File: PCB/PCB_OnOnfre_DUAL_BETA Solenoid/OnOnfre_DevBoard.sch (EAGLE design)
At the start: 31 parts, among them J1 9PIN 2.54MM, J3Y S8050, J7 8p, K1 G5Q-1-DC12, K2 G5Q-1-DC12, U2 esp12

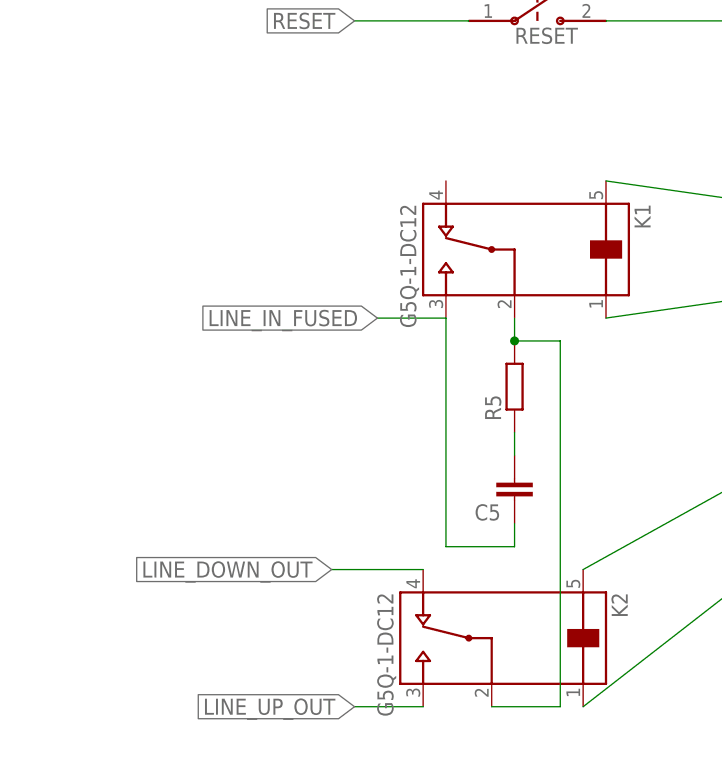
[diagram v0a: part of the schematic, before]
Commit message: estores
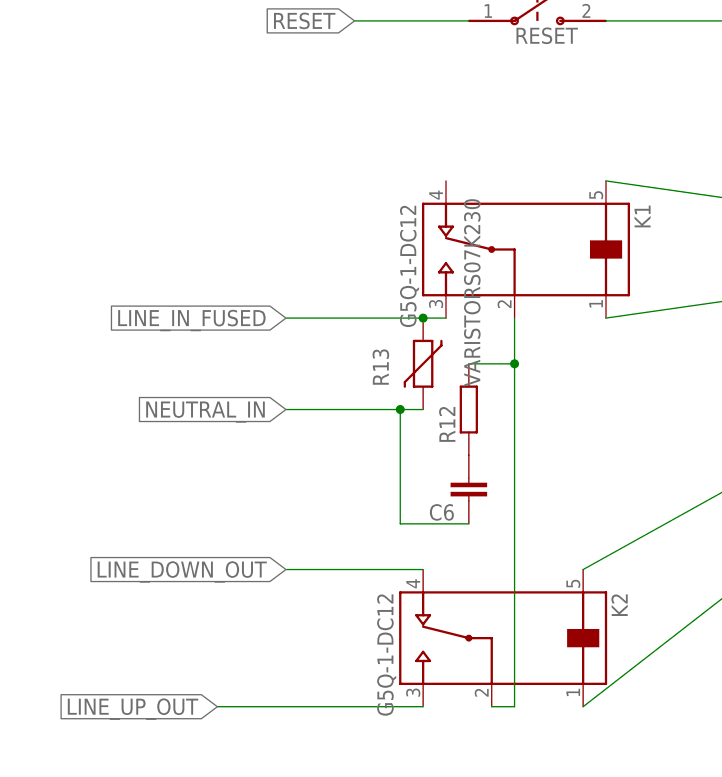
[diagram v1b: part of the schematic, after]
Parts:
- removed C5: (no value), rcl:C-EU102-043X133
- removed R5: (no value), resistor:R-EU_R2512
- added C6: (no value), rcl:C-EU102-043X133
- added R12: (no value), resistor:R-EU_R2512
- added R13: VARISTORS07K230, varistor:VARISTORS07K230
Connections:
- removed net N$4: C5.2, R5.1
- new net N$5: C6.2, R12.1
- net LINE_IN_FUSED: now also R13.1; no longer C5.1
- net N$3: now also R12.2; no longer R5.2
- net NEUTRAL_IN: now also C6.1, R13.2
